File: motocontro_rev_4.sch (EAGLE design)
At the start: 9 parts

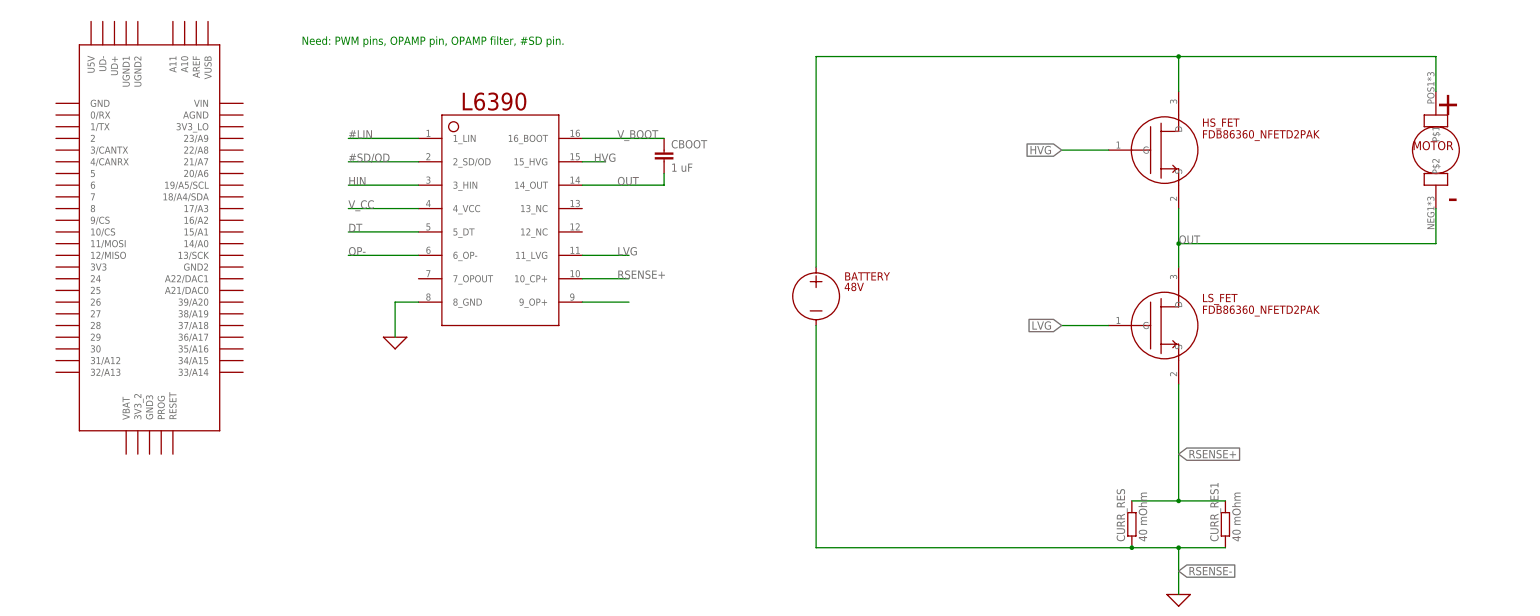
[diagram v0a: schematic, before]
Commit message: Wed. Night Progress
Lots of parts to be updated
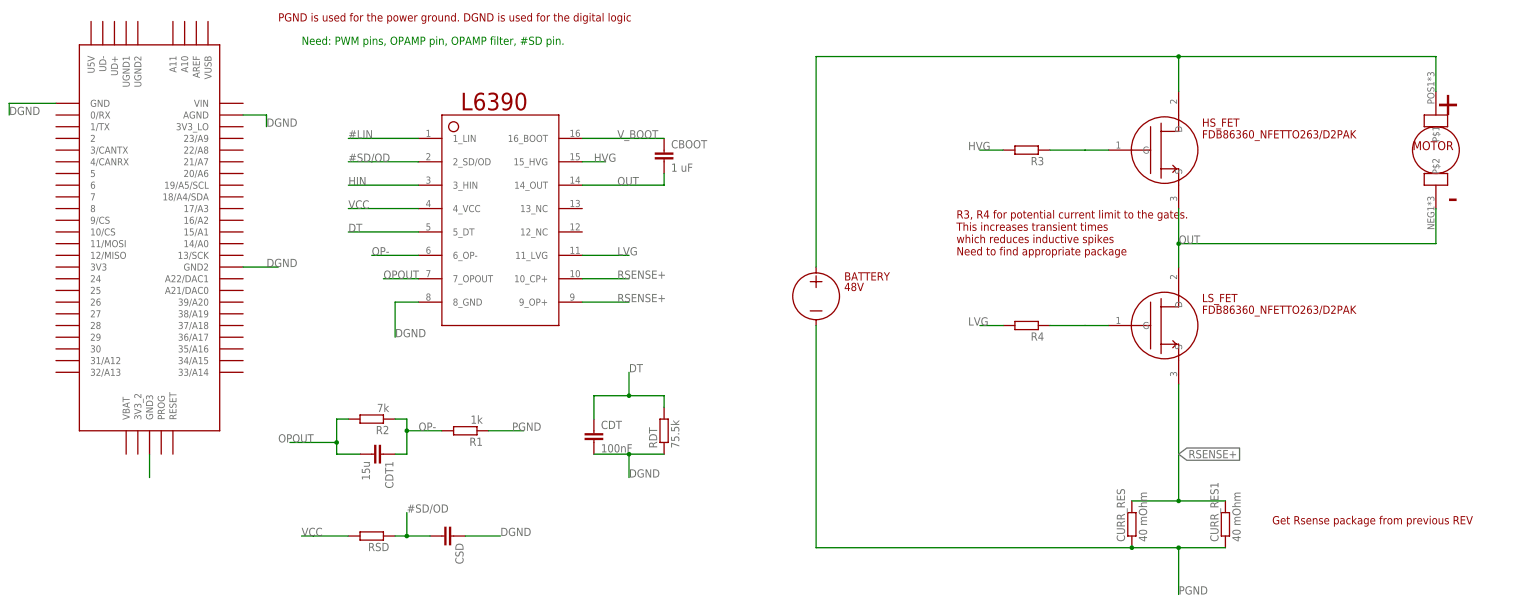
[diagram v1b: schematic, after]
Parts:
- added CDT: 100nF, eagle-ltspice:CC1206
- added CDT1: 15u, eagle-ltspice:CC1206
- added CSD: (no value), eagle-ltspice:CC1206
- added R1: 1k, eagle-ltspice:RR2012
- added R2: 7k, eagle-ltspice:RR2012
- added R3, R4, RSD: (no value), eagle-ltspice:RR2012
- added RDT: 75.5k, eagle-ltspice:RR2012
- HS_FET, LS_FET: value FDB86360_NFETD2PAK -> FDB86360_NFETTO263/D2PAK; device motocontro_rev_4:FDB86360_NFETD2PAK -> motocontro_rev_4:FDB86360_NFETTO263/D2PAK
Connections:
- removed net 0: U$1.8_GND
- removed net RSENSE-: BATTERY.-, CURR_RES.1, CURR_RES1.1
- removed net V_CC: U$1.4_VCC
- new net DGND: CDT.2, CSD.1, RDT.1, U$1.8_GND, U$2.AGND, U$2.GND, U$2.GND2
- new net N$1: U$2.GND3
- new net N$3: LS_FET.G, R4.1
- new net OPOUT: CDT1.2, R2.2, U$1.7_OPOUT
- new net PGND: BATTERY.-, CURR_RES.1, CURR_RES1.1, R1.1
- new net VCC: RSD.2, U$1.4_VCC
- net #SD/OD: now also CSD.2, RSD.1
- net DT: now also CDT.1, RDT.2
- net HVG: now also R3.2; no longer HS_FET.G
- net LVG: now also R4.2; no longer LS_FET.G
- net N$2: now also HS_FET.G, R3.1; no longer U$1.9_OP+
- net OP-: now also CDT1.1, R1.2, R2.1
- net RSENSE+: now also U$1.9_OP+
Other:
- note added: "Get Rsense package from previous REV"
- note added: "PGND is used for the power ground. DGND is used for the digital logic"
- note added: "R3, R4 for potential current limit to the gates. This increases transient times which reduces inductive spikes Need to find appropriate package"
